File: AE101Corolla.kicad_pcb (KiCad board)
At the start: 4 copper layers, 100 x 100 mm, 13 parts, among them J1 175448-6, M1 Module-mega-mcu144-0.7, M2 Module-vr-discrete-0.5, M3 Module-vr-max9924-0.1, M4 Module-power_12and5V-0.3

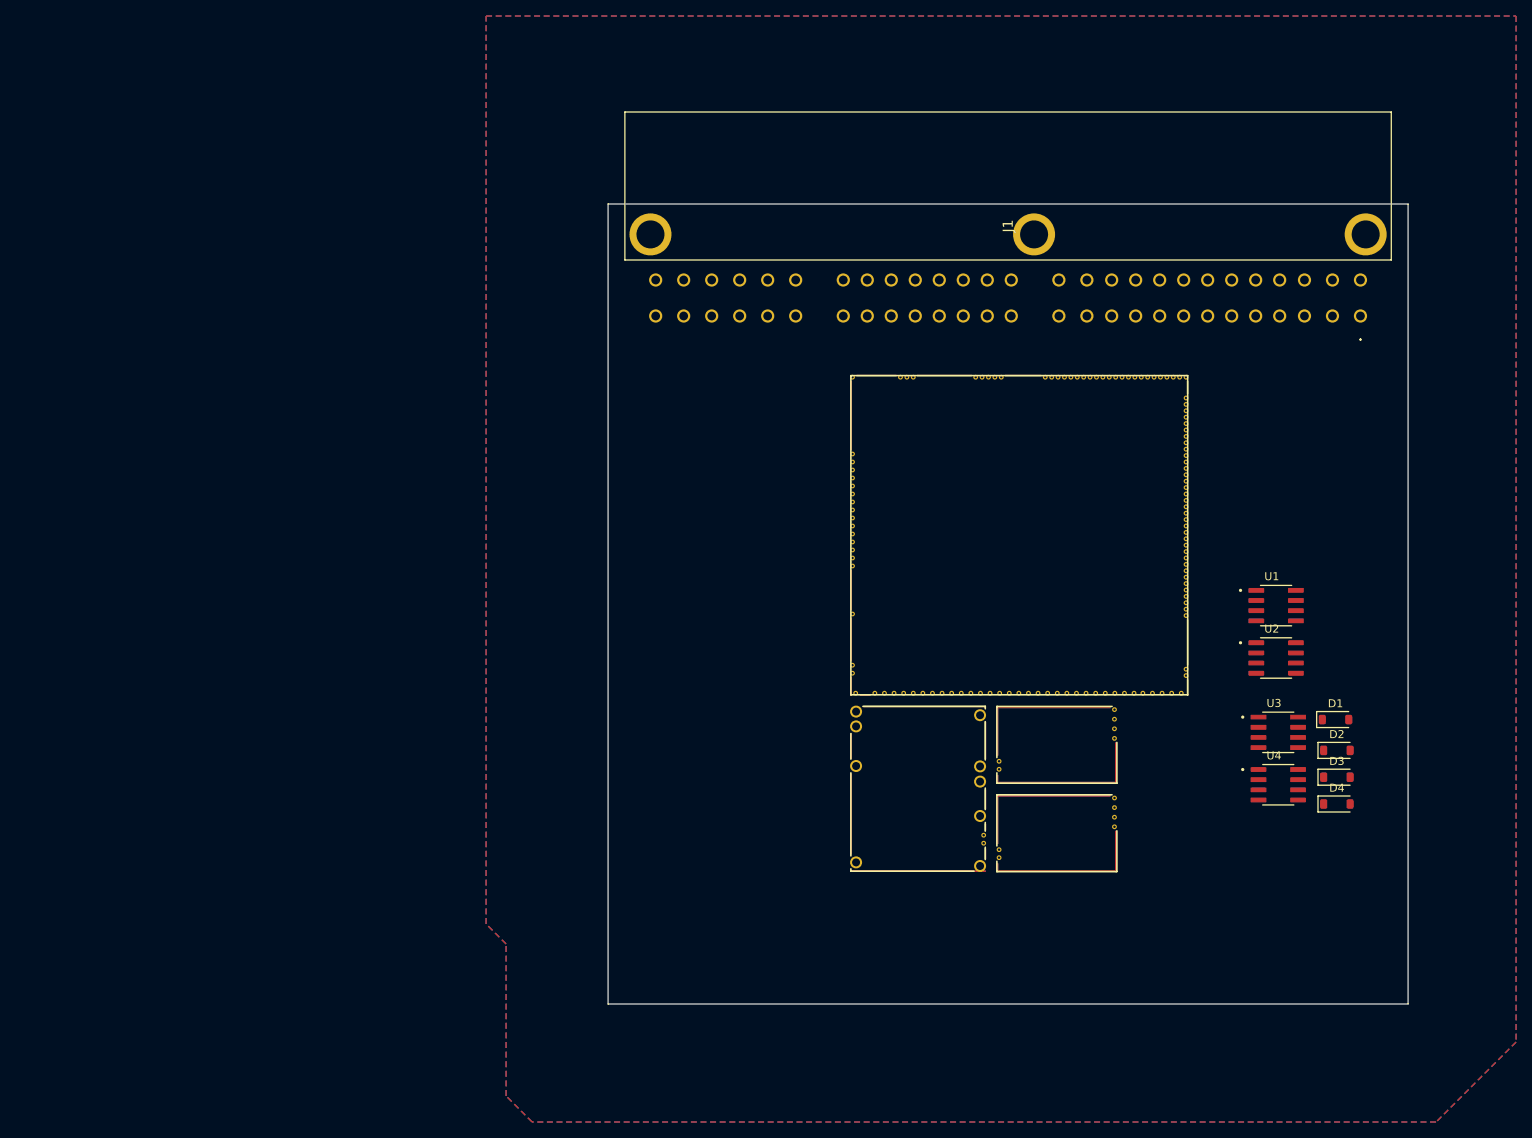
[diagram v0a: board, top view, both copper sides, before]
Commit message: sync
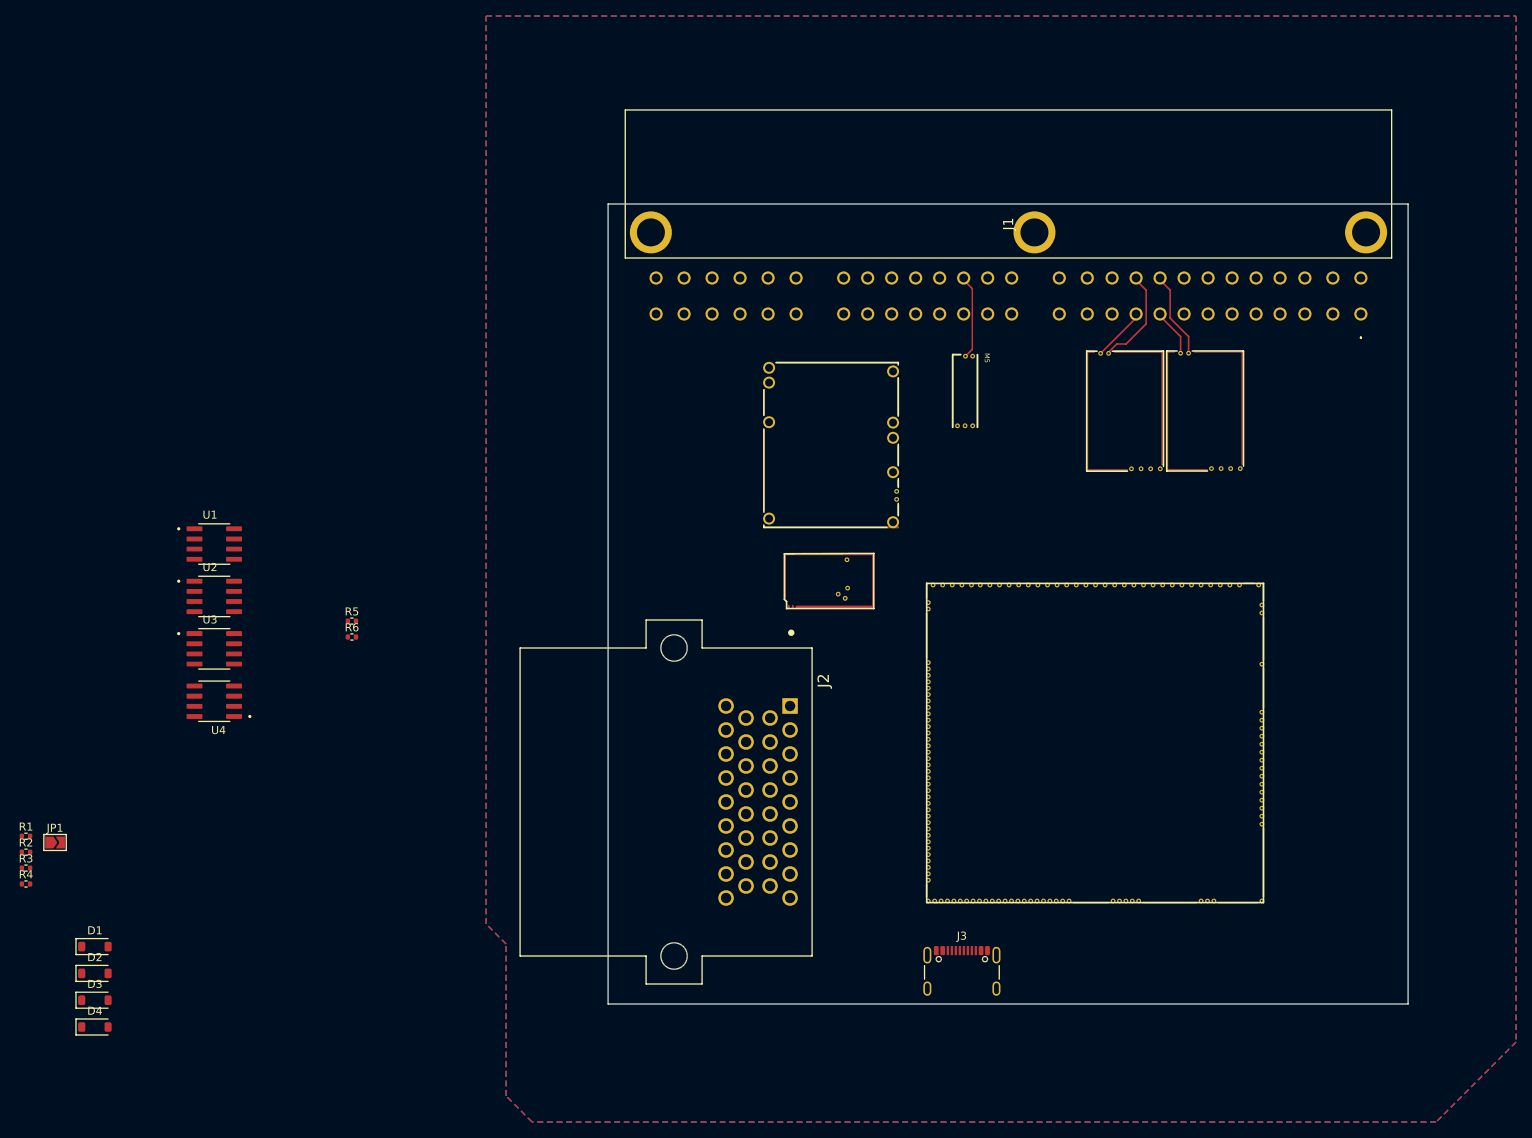
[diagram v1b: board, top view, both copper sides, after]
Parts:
- added J2: 6437288-2, 6437288_2:TE_6437288-2, F.Cu at (118.8, 124.8)
- added J3: USB_C_Receptacle_USB2.0_14P, Connector_USB:USB_C_Receptacle_GCT_USB4105-xx-A_16P_TopMnt_Horizontal, F.Cu at (144.2, 147.0)
- added JP1: SolderJumper_2_Open, Jumper:SolderJumper-2_P1.3mm_Open_TrianglePad1.0x1.5mm, F.Cu at (30.9, 129.8)
- added M5: Module-knock-0.2, knock:knock, F.Cu at (143.0, 68.7)
- added M6: Module-can-0.1, can:can, F.Cu at (121.9, 100.7)
- added R1: 4.7k, Resistor_SMD:R_0402_1005Metric, F.Cu at (27.2, 129.0)
- added R2: 4.7k, Resistor_SMD:R_0402_1005Metric, F.Cu at (27.2, 131.0)
- added R3: 4.7k, Resistor_SMD:R_0402_1005Metric, F.Cu at (27.2, 133.0)
- added R4: 4.7k, Resistor_SMD:R_0402_1005Metric, F.Cu at (27.2, 135.0)
- added R5: 5.1k, Resistor_SMD:R_0402_1005Metric, F.Cu at (68.0, 102.1)
- added R6: 5.1k, Resistor_SMD:R_0402_1005Metric, F.Cu at (68.0, 104.1)
- M1: footprint megamcu144:mega-mcu144 -> mega-mcu144:mega-mcu144
- M3: footprint vrmax9924:vr-max9924 -> vr-max9924:vr-max9924
- M4: footprint power5_12:power_12and5V -> power_12and5V:power_12and5V
- moved D2 157.7 mm to (35.8, 146.2)
- moved D3 157.7 mm to (35.8, 149.5)
- moved D4 157.7 mm to (35.8, 152.9)
- moved D1 157.7 mm to (35.8, 142.8)
- moved U3 133.4 mm to (50.8, 105.6)
- moved U4 133.4 mm to (50.8, 112.2), turned to 180 degrees
- moved U1 132.9 mm to (50.8, 92.5)
- moved U2 132.9 mm to (50.8, 99.1)
- moved M3 66.2 mm to (159.7, 68.3), turned to -90 degrees
- moved M2 58.2 mm to (169.7, 68.3), turned to -90 degrees
- moved M1 53.7 mm to (182.0, 97.3), turned to 180 degrees
- moved M4 44.3 mm to (119.4, 90.5)
- moved J1 0.25 mm to (194.1, 63.8)
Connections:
- D2 pad 2: Net-(D2-A) -> /BOOSTSOLENOID_OUT
- D3 pad 2: /IATOPEN_OUT -> /IACOPEN_OUT
- D4 pad 2: /IATCLOSE_OUT -> /IACCLOSE_OUT
- J1 pad 1: unconnected-(J1-Pad1) -> GND
- J1 pad 11: unconnected-(J1-ACT-Pad11) -> /ACTEMP
- J1 pad 13: unconnected-(J1-FC-Pad13) -> /FUELRELAY_OUT
- J1 pad 15: unconnected-(J1-BATT-Pad15) -> +12V_PERM
- J1 pad 16: unconnected-(J1-+B1-Pad16) -> +12V_RAW
- J1 pad 17: unconnected-(J1-ELS-Pad17) -> /ELECTRICLOAD
- J1 pad 18: unconnected-(J1-SPD-Pad18) -> /SPEED
- J1 pad 19: unconnected-(J1-AC1-Pad19) -> /ACSTATUS
- J1 pad 2: unconnected-(J1-Pad2) -> /INJ1_OUT
- J1 pad 21: unconnected-(J1-W?-Pad21) -> /CHECKENGINE
- J1 pad 22: unconnected-(J1-+B-Pad22) -> +12V_RAW
- J1 pad 23: unconnected-(J1-Pad23) -> /IACOPEN_OUT
- J1 pad 24: unconnected-(J1-Pad24) -> /IACCLOSE_OUT
- J1 pad 28: unconnected-(J1-Pad28) -> /SYNC+
- J1 pad 29: unconnected-(J1-Pad29) -> /VR+
- J1 pad 32: unconnected-(J1-Pad32) -> /IGN1
- J1 pad 36: unconnected-(J1-Pad36) -> /SYNC-
- J1 pad 37: unconnected-(J1-Pad37) -> /VR-
- J1 pad 41: unconnected-(J1-Pad41) -> /NARROWO2_UPSTR
- J1 pad 42: unconnected-(J1-Pad42) -> /NARROWO2_DOWNSTR
- J1 pad 43: unconnected-(J1-Pad43) -> /CLT
- J1 pad 44: unconnected-(J1-Pad44) -> /IAT
- J1 pad 45: unconnected-(J1-Pad45) -> /MAP
- J1 pad 47: unconnected-(J1-Pad47) -> GND
- J1 pad 49: unconnected-(J1-Pad49) -> /KNOCK_RAW
- J1 pad 51: unconnected-(J1-Pad51) -> /IDLSW
- J1 pad 52: unconnected-(J1-Pad52) -> +5VP
- J1 pad 53: unconnected-(J1-Pad53) -> /TPS
- J1 pad 54: unconnected-(J1-Pad54) -> GNDA
- J1 pad 6: unconnected-(J1-Pad6) -> GND
- J1 pad 7: unconnected-(J1-Pad7) -> /INJ3_OUT
- J1 pad 8: unconnected-(J1-Pad8) -> GND
- J1 pad 9: unconnected-(J1-Pad9) -> /NEUTRALSW
- M1 pad E1: unconnected-(M1-SPI2_SCK/CAN2_TX-PadE1) -> Net-(M1-SPI2_SCK/CAN2_TX)
- M1 pad E16: unconnected-(M1-OUT_PWM3-PadE16) -> /BOOSTSOLENOID_IN
- M1 pad E17: unconnected-(M1-OUT_PWM2-PadE17) -> /IACOPEN_IN
- M1 pad E27: unconnected-(M1-OUT_PWM1-PadE27) -> /IACCLOSE_IN
- M1 pad E28: unconnected-(M1-OUT_PWM8-PadE28) -> /VR_THRESH
- M1 pad E31: unconnected-(M1-OUT_INJ5-PadE31) -> /FUELRELAY_IN
- M1 pad E38: unconnected-(M1-V5A_SWITCHABLE-PadE38) -> +5VA
- M1 pad E4: unconnected-(M1-SPI2_CS/CAN2_RX-PadE4) -> Net-(M1-SPI2_CS/CAN2_RX)
- M1 pad N2: unconnected-(M1-USBM-PadN2) -> /USB-
- M1 pad N26: unconnected-(M1-IN_VIGN-PadN26) -> /VIGN
- M1 pad N27: unconnected-(M1-VBAT-PadN27) -> /VBAT
- M1 pad N28: unconnected-(M1-V33_SWITCHABLE-PadN28) -> +3.3VA
- M1 pad N29: unconnected-(M1-OUT_PWR_EN-PadN29) -> /5VP_ENABLE
- M1 pad N3: unconnected-(M1-USBP-PadN3) -> /USB+
- M1 pad N31: unconnected-(M1-VCC-PadN31) -> +5V
- M1 pad N4: unconnected-(M1-VBUS-PadN4) -> Net-(M1-VBUS)
- M1 pad S1: unconnected-(M1-IN_D4-PadS1) -> /IDLSW
- M1 pad S10: unconnected-(M1-IN_AUX4-PadS10) -> /AUX4
- M1 pad S11: unconnected-(M1-IN_AUX3-PadS11) -> /AUX3
- M1 pad S12: unconnected-(M1-IN_AUX2-PadS12) -> /AUX2
- M1 pad S13: unconnected-(M1-IN_AUX1-PadS13) -> /AUX1
- M1 pad S14: unconnected-(M1-IN_RES2-PadS14) -> /RES2
- M1 pad S15: unconnected-(M1-IN_O2S2-PadS15) -> /NARROWO2_DOWNSTR
- M1 pad S16: unconnected-(M1-IN_O2S-PadS16) -> /NARROWO2_UPSTR
- M1 pad S17: unconnected-(M1-IN_RES1-PadS17) -> /RES1
- M1 pad S18: unconnected-(M1-IN_RES3-PadS18) -> /RES3
- M1 pad S2: unconnected-(M1-IN_D3-PadS2) -> /ACSTATUS
- M1 pad S21: unconnected-(M1-IN_MAP1-PadS21) -> /MAP
- M1 pad S22: unconnected-(M1-IN_CRANK-PadS22) -> /MAINVR_OUT
- M1 pad S23: unconnected-(M1-IN_KNOCK-PadS23) -> /KNOCK_PROCESSED
- M1 pad S24: unconnected-(M1-IN_CAM-PadS24) -> /SYNCVR_OUT
- M1 pad S25: unconnected-(M1-IN_VSS-PadS25) -> /SPEED
- M1 pad S26: unconnected-(M1-IN_IAT-PadS26) -> /IAT
- M1 pad S28: unconnected-(M1-IN_CLT-PadS28) -> /CLT
- M1 pad S3: unconnected-(M1-IN_D2-PadS3) -> /ELECTRICLOAD
- M1 pad S30: unconnected-(M1-IN_TPS-PadS30) -> /TPS
- M1 pad S35: unconnected-(M1-VREF1-PadS35) -> /VREF1
- M1 pad W1: unconnected-(M1-GNDA-PadW1) -> GNDA
- M1 pad W10: unconnected-(M1-IGN2-PadW10) -> /IGN2
- M1 pad W11: unconnected-(M1-IGN1-PadW11) -> /IGN1
- M1 pad W12: unconnected-(M1-CANH-PadW12) -> /CAN1H
- M1 pad W13: unconnected-(M1-CANL-PadW13) -> /CAN1L
- M1 pad W8: unconnected-(M1-IGN4-PadW8) -> /IGN4
- M1 pad W9: unconnected-(M1-IGN3-PadW9) -> /IGN3
- M2 pad E1: unconnected-(M2-Thresh_IN-PadE1) -> /VR_THRESH
- M2 pad E3: unconnected-(M2-OUT-PadE3) -> /SYNCVR_OUT
- M2 pad E4: unconnected-(M2-V5_IN-PadE4) -> +5VA
- M2 pad G: unconnected-(M2-GND-PadG) -> GND
- M2 pad W1: unconnected-(M2-VR--PadW1) -> /SYNC-
- M2 pad W2: unconnected-(M2-VR+-PadW2) -> /SYNC+
- M3 pad E1: unconnected-(M3-HALL_EN-PadE1) -> Net-(JP1-A)
- M3 pad E3: unconnected-(M3-OUT-PadE3) -> /MAINVR_OUT
- M3 pad E4: unconnected-(M3-V5_IN-PadE4) -> +5VA
- M3 pad G: unconnected-(M3-GND-PadG) -> GND
- M3 pad W1: unconnected-(M3-VR-/HALL-PadW1) -> /VR-
- M3 pad W2: unconnected-(M3-VR+-PadW2) -> /VR+
- M4 pad E1: unconnected-(M4-VBAT-PadE1) -> /VBAT
- M4 pad E3: unconnected-(M4-VIGN-PadE3) -> /VIGN
- M4 pad E4: unconnected-(M4-V5-PadE4) -> +5V
- M4 pad E5: unconnected-(M4-EN_5VP-PadE5) -> /5VP_ENABLE
- M4 pad S1: unconnected-(M4-GND-PadS1) -> GND
- M4 pad V1: unconnected-(M4-V12_PERM-PadV1) -> +12V_PERM
- M4 pad V2: unconnected-(M4-IN_VIGN-PadV2) -> +12V_RAW
- M4 pad V3: unconnected-(M4-V12_RAW-PadV3) -> +12V_RAW
- M4 pad V4: unconnected-(M4-5VP-PadV4) -> +5VP
- U3 pad 1: unconnected-(U3-IN1-Pad1) -> /BOOSTSOLENOID_IN
- U3 pad 5: /FUELRELAY_OUT -> GND
- U3 pad 6: unconnected-(U3-DRAIN2-Pad6) -> /FUELRELAY_OUT
- U3 pad 7: Net-(D2-A) -> GND
- U3 pad 8: unconnected-(U3-DRAIN1-Pad8) -> /BOOSTSOLENOID_OUT
- U4 pad 1: /IATCLOSE_IN -> /IACCLOSE_IN
- U4 pad 3: /IATOPEN_IN -> /IACOPEN_IN
- U4 pad 5: /IATOPEN_OUT -> GND
- U4 pad 6: unconnected-(U4-DRAIN2-Pad6) -> /IACOPEN_OUT
- U4 pad 7: /IATCLOSE_OUT -> GND
- U4 pad 8: unconnected-(U4-DRAIN1-Pad8) -> /IACCLOSE_OUT
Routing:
- net /VR-: track 0.00 -> 12.3 mm
- net /SYNC-: track 0.00 -> 10.6 mm
- net /KNOCK_RAW: track 0.00 -> 10.3 mm
- net /VR+: track 0.00 -> 6.51 mm
- net /SYNC+: track 0.00 -> 5.71 mm
- net +12V_RAW: track 0.00 -> 4.50 mm
